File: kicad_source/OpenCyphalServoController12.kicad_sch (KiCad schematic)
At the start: 49 parts, among them CN1 RASPBERRYPI_PICO, CN11 CONN_02X03, CN12 Conn_01x03, CN2 SM04B-SRSS-TB, CN3 SM04B-SRSS-TB, CN6 691322310002, CN7 CONN_02X03, CN8 Conn_02x08_Odd_Even, SW1 SPST, U3 24LC64

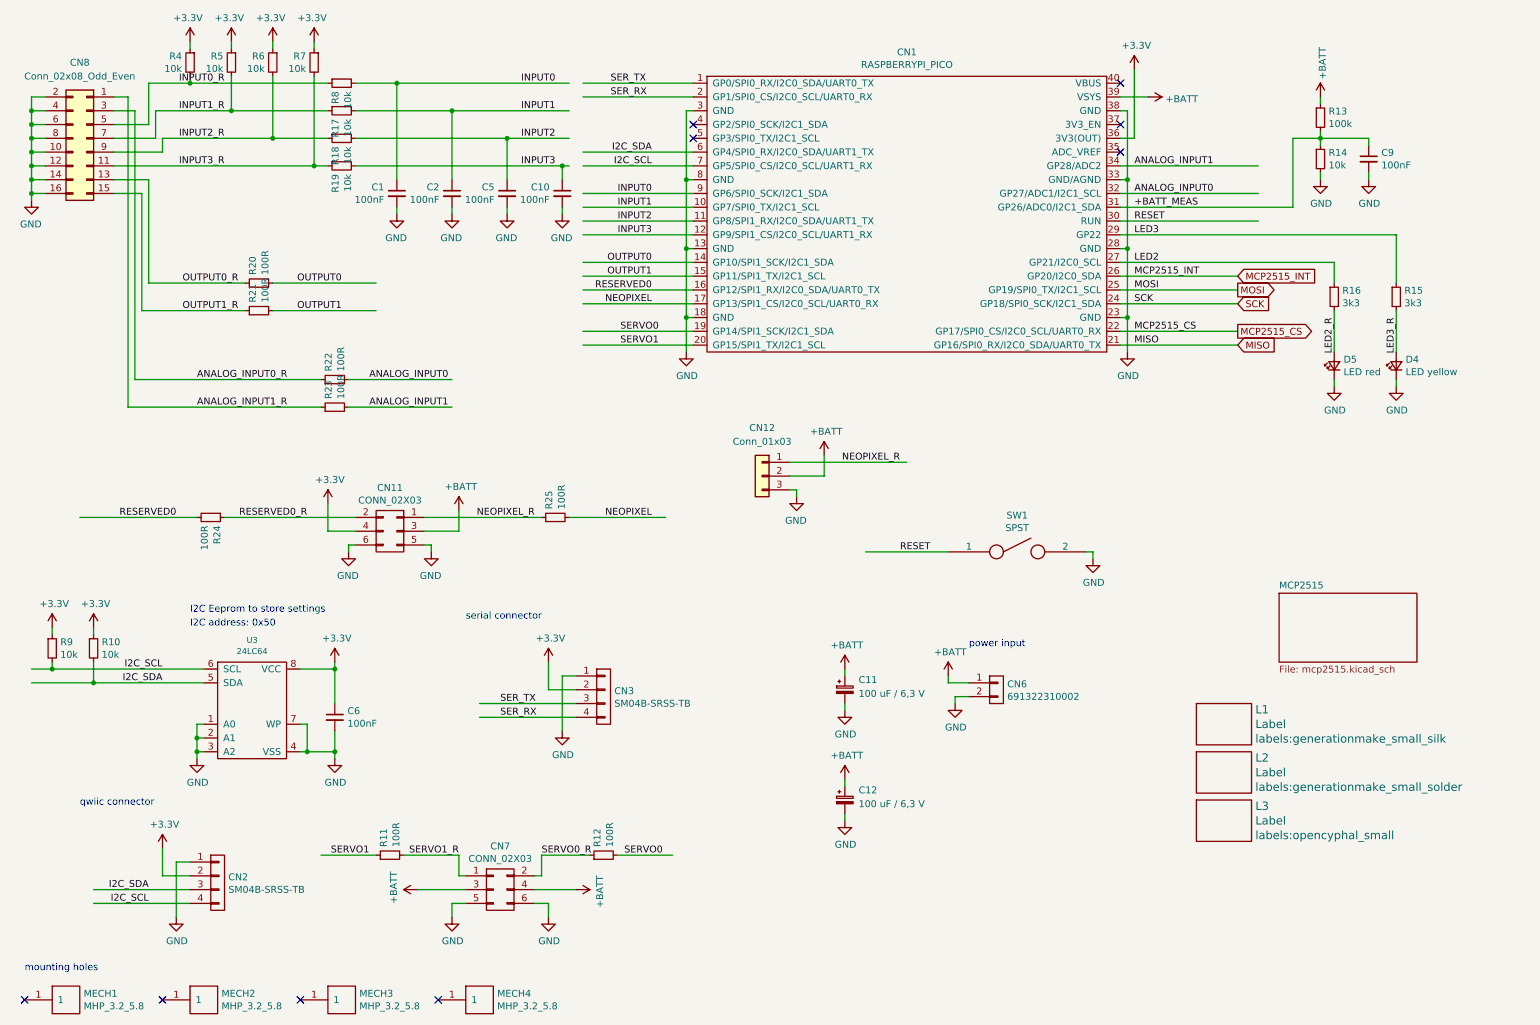
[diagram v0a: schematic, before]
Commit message: reworked schematic
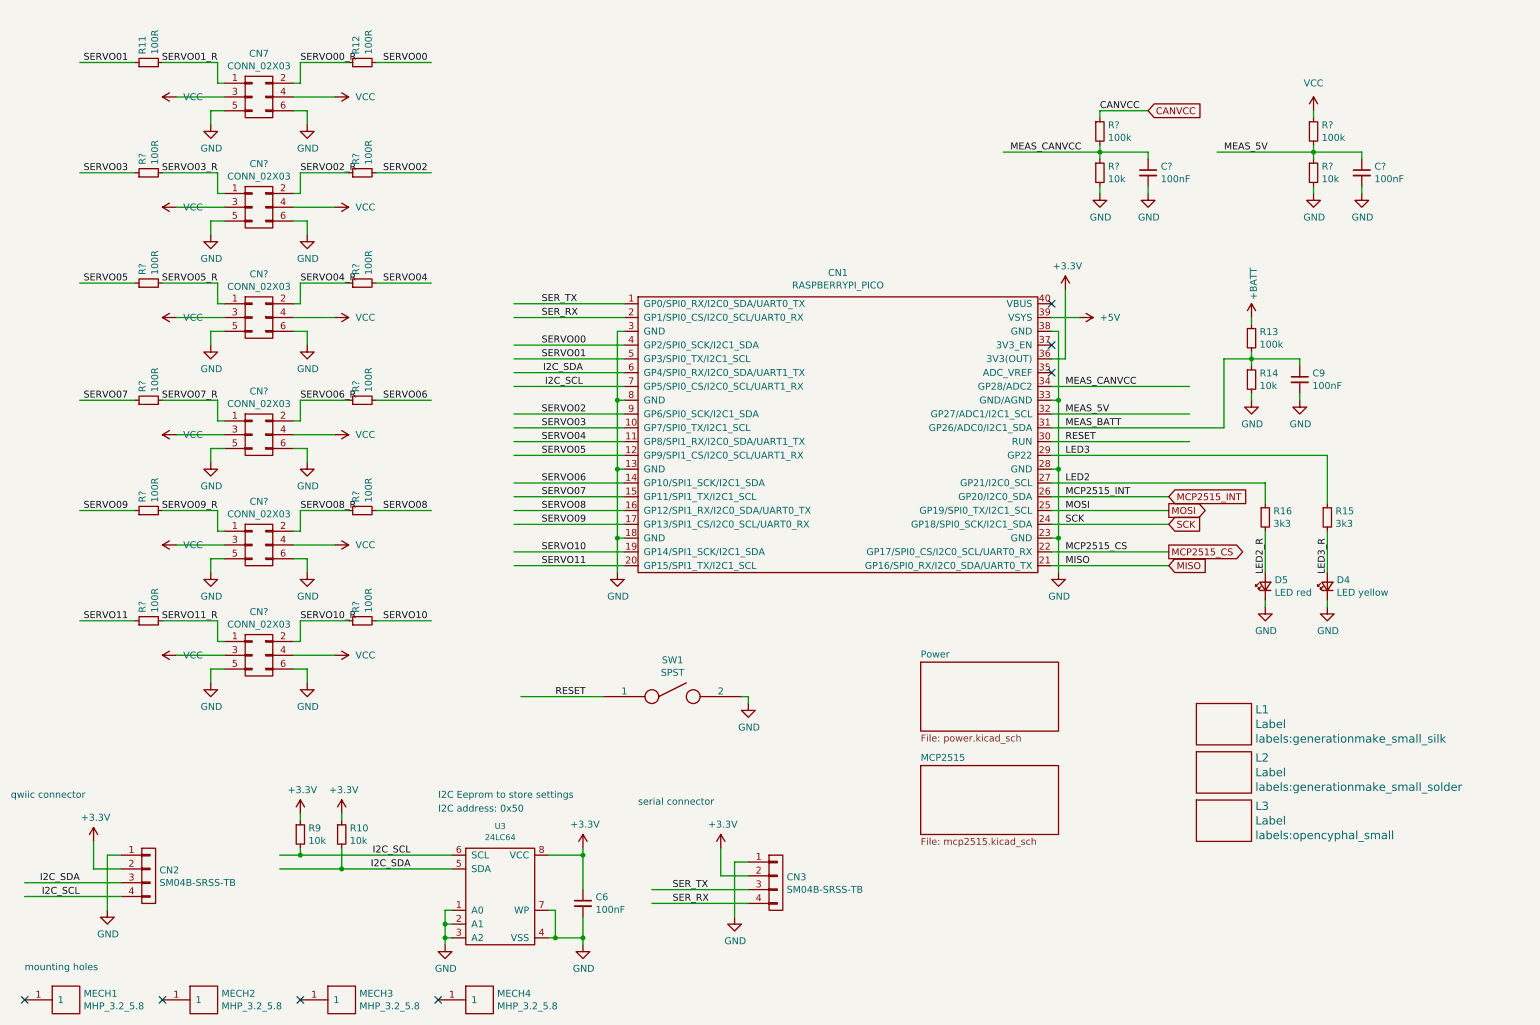
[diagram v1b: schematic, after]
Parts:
- removed C1, C10, C2, C5: 100nF, Capacitor_SMD:C_0603_1608Metric, symbol Device:C_Small
- removed C11, C12: 100 uF / 6,3 V, Capacitor_SMD:CP_Elec_5x5.3, symbol Device:C_Polarized_Small
- removed CN11: CONN_02X03, Connector_PinHeader_2.54mm:PinHeader_2x03_P2.54mm_Vertical, symbol OpenCyphalPicoBase-rescue:CONN_02X03-mechanical-connectors
- removed CN12: Conn_01x03, Connector_JST:JST_PH_S3B-PH-SM4-TB_1x03-1MP_P2.00mm_Horizontal, symbol Connector_Generic:Conn_01x03
- removed CN6: 691322310002, CON_wuerth:WR-TBL_691322310002, symbol OpenCyphalPicoBase-rescue:CONN_01X02-mechanical-connectors
- removed CN8: Conn_02x08_Odd_Even, Connector_PinHeader_2.54mm:PinHeader_2x08_P2.54mm_Vertical, symbol Connector_Generic:Conn_02x08_Odd_Even
- removed R17, R18, R19, R4, R5, R6, R7, R8: 10k, Resistor_SMD:R_0603_1608Metric, symbol Device:R_Small
- removed R20, R21, R22, R23, R24, R25: 100R, Resistor_SMD:R_0603_1608Metric, symbol Device:R_Small
- added C? (x2): 100nF, Capacitor_SMD:C_0603_1608Metric, symbol Device:C_Small
- added CN? (x5): CONN_02X03, Connector_PinHeader_2.54mm:PinHeader_2x03_P2.54mm_Horizontal, symbol OpenCyphalPicoBase-rescue:CONN_02X03-mechanical-connectors
- added R? (x10): 100R, Resistor_SMD:R_0603_1608Metric, symbol Device:R_Small
- added R? (x2): 10k, Resistor_SMD:R_0603_1608Metric, symbol Device:R_Small
- added R? (x2): 100k, Resistor_SMD:R_0603_1608Metric, symbol Device:R_Small
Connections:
- net +BATT: no longer CN1.39 (VSYS), CN7.3 (P3), CN7.4 (P4)
- net GND: now also C?.2, C?.2, CN?.5 (P5), CN?.5 (P5), CN?.5 (P5), CN?.5 (P5), CN?.5 (P5), CN?.6 (P6), CN?.6 (P6), CN?.6 (P6), CN?.6 (P6), CN?.6 (P6), R?.2, R?.2
- net SERVO00: now reaches CN1.4 (GP2/SPI0_SCK/I2C1_SDA)
- net SERVO00: now also R12.2
- net SERVO01: now reaches CN1.5 (GP3/SPI0_TX/I2C1_SCL)
- net SERVO01: now also R11.1
- net +BATT_MEAS renamed MEAS_BATT
- net ANALOG_INPUT0 renamed MEAS_5V
- net MEAS_5V: now also C?.1, R?.1, R?.2
- net ANALOG_INPUT1 renamed MEAS_CANVCC
- net MEAS_CANVCC: now also C?.1, R?.1, R?.2
- net INPUT0 renamed SERVO02
- net SERVO02: now also R?.2
- net INPUT1 renamed SERVO03
- net SERVO03: now also R?.1
- net INPUT2 renamed SERVO04
- net SERVO04: now also R?.2
- net INPUT3 renamed SERVO05
- net SERVO05: now also R?.1
- net NEOPIXEL renamed SERVO09
- net SERVO09: now also R?.1
- net OUTPUT0 renamed SERVO06
- net SERVO06: now also R?.2
- net OUTPUT1 renamed SERVO07
- net SERVO07: now also R?.1
- net RESERVED0 renamed SERVO08
- net SERVO08: now also R?.2
- net SERVO0 renamed SERVO10
- net SERVO10: now also R?.2; no longer R12.2
- net SERVO0_R renamed SERVO00_R
- net SERVO1 renamed SERVO11
- net SERVO11: now also R?.1; no longer R11.1
- net SERVO1_R renamed SERVO01_R
- new net +5V: CN1.39 (VSYS)
- new net CANVCC: R?.1
- new net SERVO02_R: CN?.2 (P2), R?.1
- new net SERVO03_R: CN?.1 (P1), R?.2
- new net SERVO04_R: CN?.2 (P2), R?.1
- new net SERVO05_R: CN?.1 (P1), R?.2
- new net SERVO06_R: CN?.2 (P2), R?.1
- new net SERVO07_R: CN?.1 (P1), R?.2
- new net SERVO08_R: CN?.2 (P2), R?.1
- new net SERVO09_R: CN?.1 (P1), R?.2
- new net SERVO10_R: CN?.2 (P2), R?.1
- new net SERVO11_R: CN?.1 (P1), R?.2
- new net VCC: CN7.3 (P3), CN7.4 (P4), CN?.3 (P3), CN?.3 (P3), CN?.3 (P3), CN?.3 (P3), CN?.3 (P3), CN?.4 (P4), CN?.4 (P4), CN?.4 (P4), CN?.4 (P4), CN?.4 (P4), R?.1
- no-connect marks 9 -> 7
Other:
- added sheet Power (power.kicad_sch)
- note removed: "power input"
- title: OpenCyphalPicoBase -> OpenCyphalServoController12
- moved on the sheet: C6, C9, CN1, CN2, CN3, CN7, D4, D5, R10, R11, R12, R13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
